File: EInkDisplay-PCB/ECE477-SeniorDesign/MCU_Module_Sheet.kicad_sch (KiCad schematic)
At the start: 20 parts, among them SW1 SW_Push_Dual_x2, U3 STM32L496ZGTxP

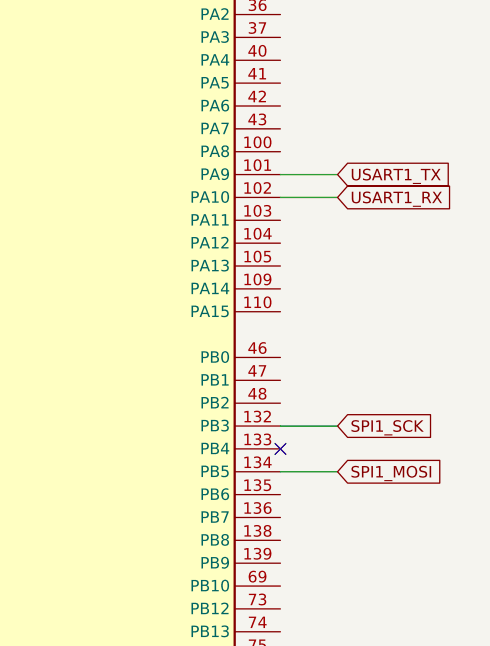
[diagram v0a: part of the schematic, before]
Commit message: push
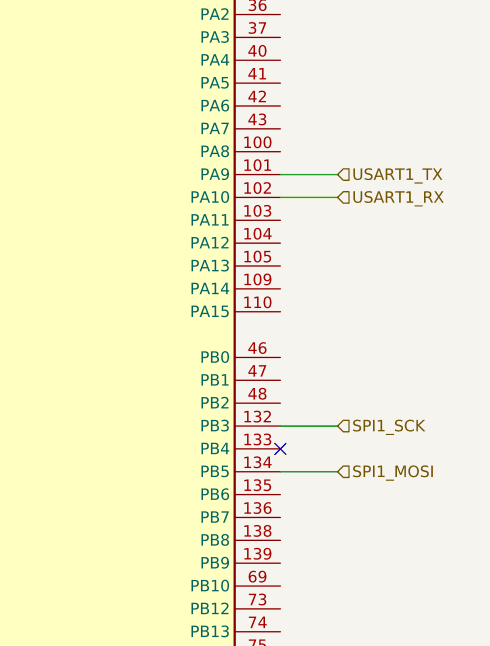
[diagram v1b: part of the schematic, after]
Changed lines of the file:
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@@
 		)
 	)
-	(global_label "USART1_RX"
+	(hierarchical_label "SPI1_MOSI"
 		(shape input)
-		(at 238.76 80.01 0)
-		(fields_autoplaced yes)
+		(at 238.76 110.49 0)
 		(effects
 			(font
@@
 			(justify left)
 		)
-		(property "Intersheetrefs" "${INTERSHEET_REFS}"
-			(at 252.268 80.01 0)
-			(effects
-				(font
-					(size 1.27 1.27)
-				)
-				(justify left)
-				(hide yes)
-			)
-		)
 	)
-	(global_label "SPI1_SCK"
+	(hierarchical_label "USART1_RX"
 		(shape input)
-		(at 238.76 105.41 0)
-		(fields_autoplaced yes)
+		(at 238.76 80.01 0)
 		(effects
 			(font
@@
 			(justify left)
 		)
-		(property "Intersheetrefs" "${INTERSHEET_REFS}"
-			(at 250.7561 105.41 0)
-			(effects
-				(font
-					(size 1.27 1.27)
-				)
-				(justify left)
-				(hide yes)
-			)
-		)
 	)
-	(global_label "SPI1_MOSI"
+	(hierarchical_label "SPI1_SCK"
 		(shape input)
-		(at 238.76 110.49 0)
-		(fields_autoplaced yes)
+		(at 238.76 105.41 0)
 		(effects
 			(font
@@
 			(justify left)
 		)
-		(property "Intersheetrefs" "${INTERSHEET_REFS}"
-			(at 251.6028 110.49 0)
-			(effects
-				(font
-					(size 1.27 1.27)
-				)
-				(justify left)
-				(hide yes)
-			)
-		)
 	)
-	(global_label "USART1_TX"
+	(hierarchical_label "USART1_TX"
 		(shape input)
 		(at 238.76 77.47 0)
-		(fields_autoplaced yes)
 		(effects
 			(font
@@
 			(justify left)
 		)
-		(property "Intersheetrefs" "${INTERSHEET_REFS}"
-			(at 251.9656 77.47 0)
-			(effects
-				(font
-					(size 1.27 1.27)
-				)
-				(justify left)
-				(hide yes)
-			)
-		)
 	)
